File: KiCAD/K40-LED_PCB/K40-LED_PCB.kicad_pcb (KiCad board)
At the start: 2 copper layers, 106.9 x 56.9 mm, 10 parts, among them J2 54-00166, U1 LDD_350HS

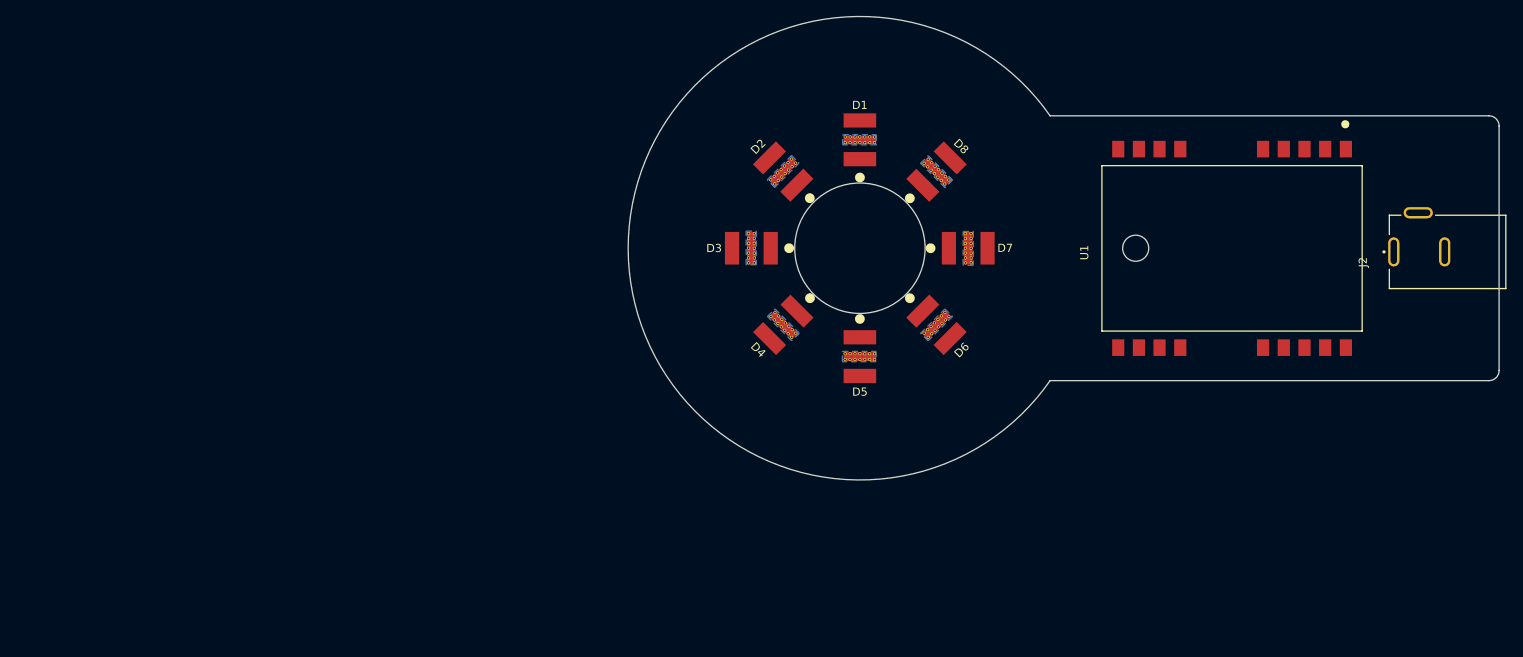
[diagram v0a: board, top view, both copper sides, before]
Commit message: Finalizing PCB. Get Checked.
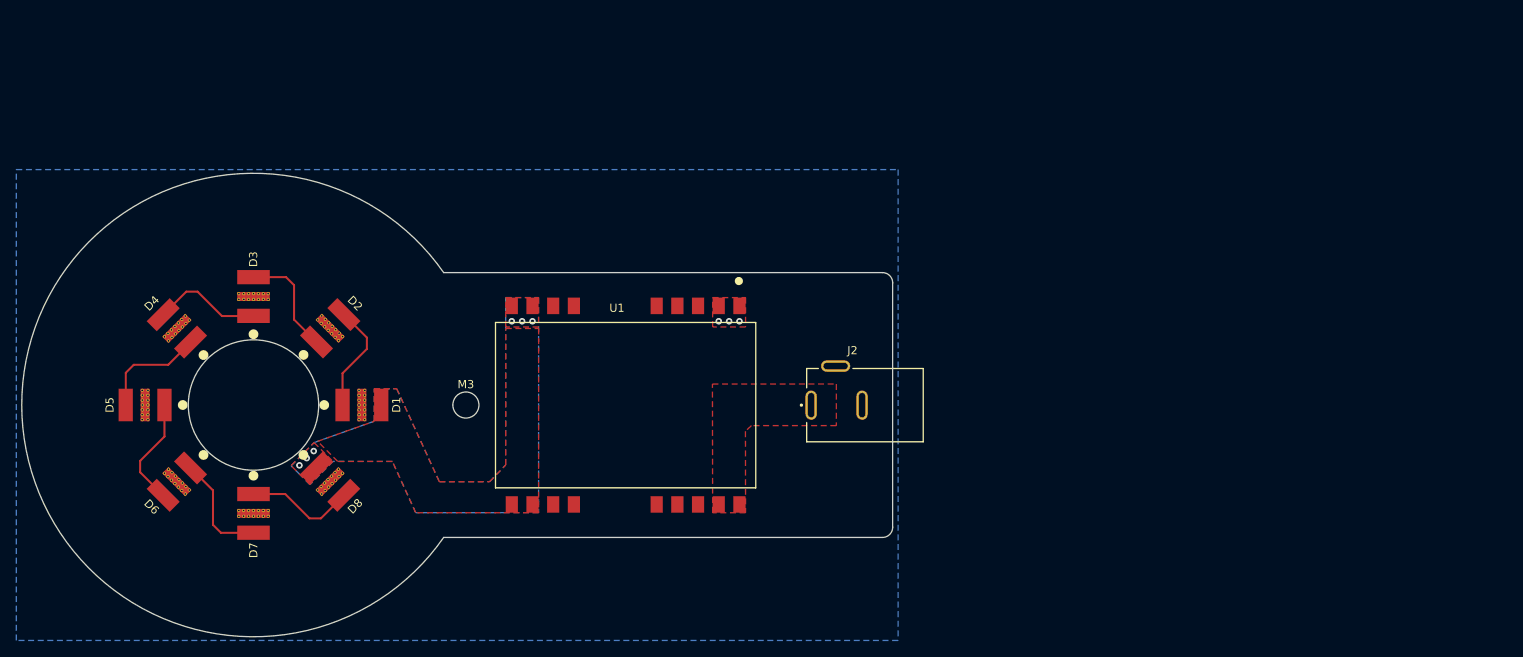
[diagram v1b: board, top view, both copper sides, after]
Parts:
- added M3: MountingHole_3.2mm_M3, MountingHole:MountingHole_3.2mm_M3, F.Cu at (148.5, 91.8)
- moved D6 95.2 mm to (113.0, 101.2), turned to 45 degrees
- moved D7 93.6 mm to (122.4, 105.1), turned to 90 degrees
- moved D5 87.9 mm to (109.1, 91.8), turned to 0 degrees
- moved D8 83.6 mm to (131.8, 101.2), turned to 135 degrees
- moved U1 76.9 mm to (186.5, 79.6)
- moved D4 74.4 mm to (113.0, 82.4), turned to -45 degrees
- moved J2 73.9 mm to (197.1, 91.8)
- moved D1 69.2 mm to (135.7, 91.8), turned to 180 degrees
- moved D3 61.4 mm to (122.4, 78.5), turned to -90 degrees
- moved D2 58.8 mm to (131.8, 82.4), turned to -135 degrees
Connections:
- D1 pad 65: (no net) -> Earth
- D2 pad 65: (no net) -> Earth
- D3 pad 65: (no net) -> Earth
- D4 pad 65: (no net) -> Earth
- D5 pad 65: (no net) -> Earth
- D6 pad 65: (no net) -> Earth
- D7 pad 65: (no net) -> Earth
- D8 pad 65: (no net) -> Earth
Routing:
- net Net-(D3-PadC): track 0.00 -> 13.5 mm
- net Net-(D1-PadC): track 0.00 -> 13.5 mm
- net Net-(D2-PadC): track 0.00 -> 13.5 mm
- net Net-(D6-PadC): track 0.00 -> 13.5 mm
- net Net-(D4-PadC): track 0.00 -> 13.5 mm
- net Net-(D5-PadC): track 0.00 -> 13.5 mm
- net Net-(D7-PadC): track 0.00 -> 13.5 mm
- net Earth: vias 0 -> 3
- net -Led: vias 0 -> 6
- added copper zone on F.Cu, net +Led
- added copper zone on F.Cu, net -Led
- added copper zone on B.Cu, net Earth
- added copper zone on F.Cu, net Earth
- added copper zone on F.Cu, net VIn
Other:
- outline, holes or cut-outs redrawn
- board text added: "PCB3D_BR_K40PositionalGuide"
- board text added: "PCB3D_TL_K40PositionalGuide"
